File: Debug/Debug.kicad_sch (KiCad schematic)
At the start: 54 parts

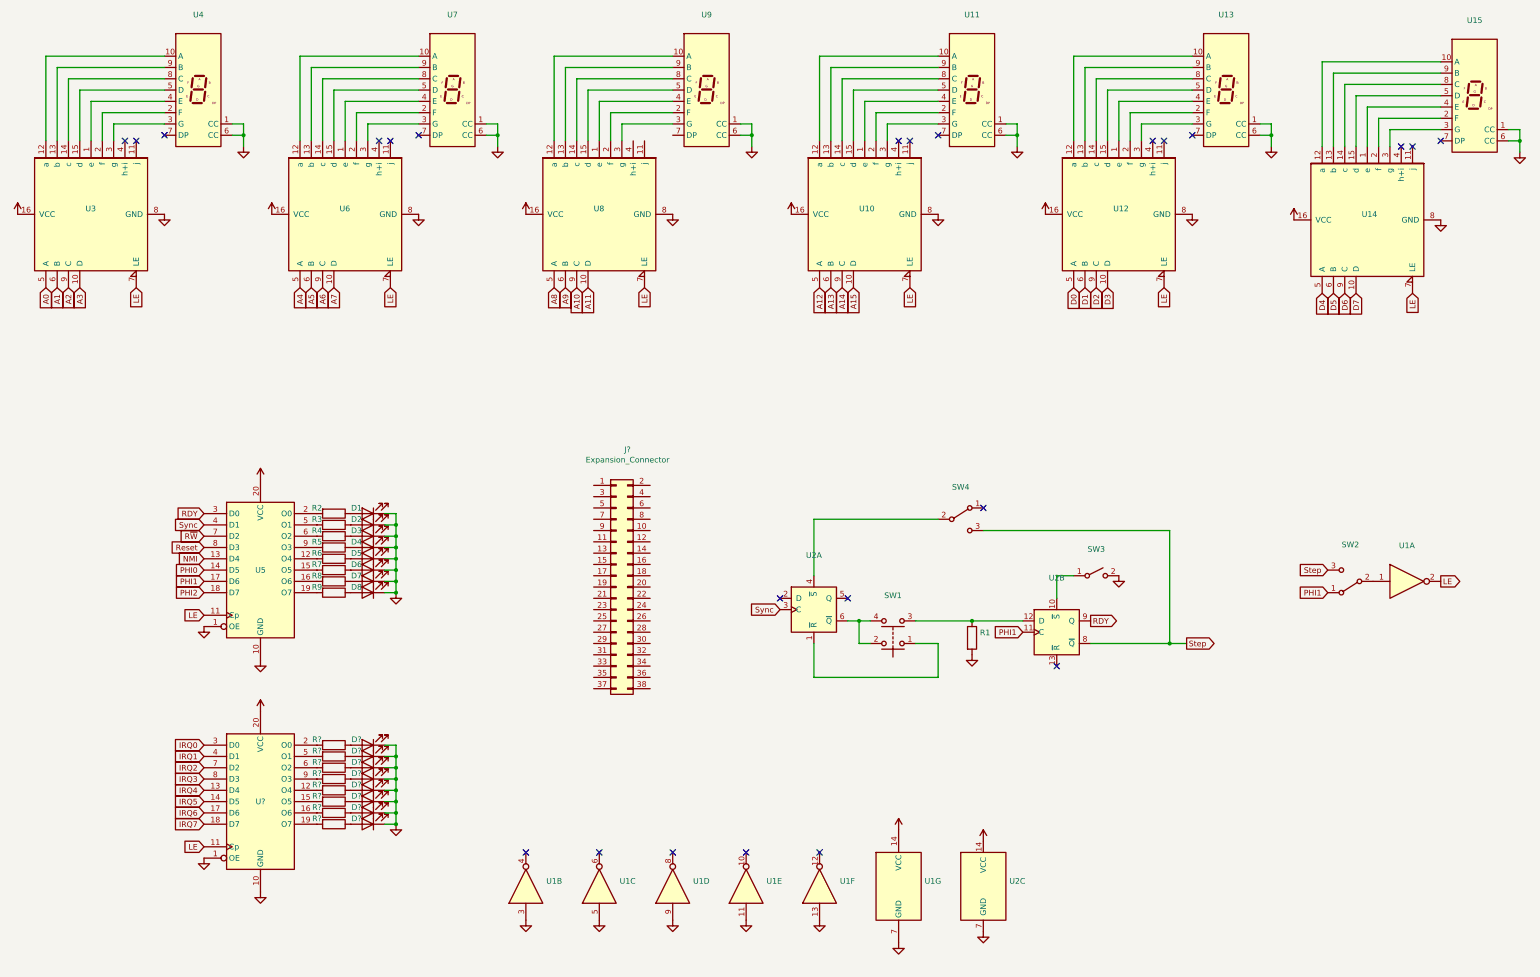
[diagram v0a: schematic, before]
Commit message: Updated debug card...
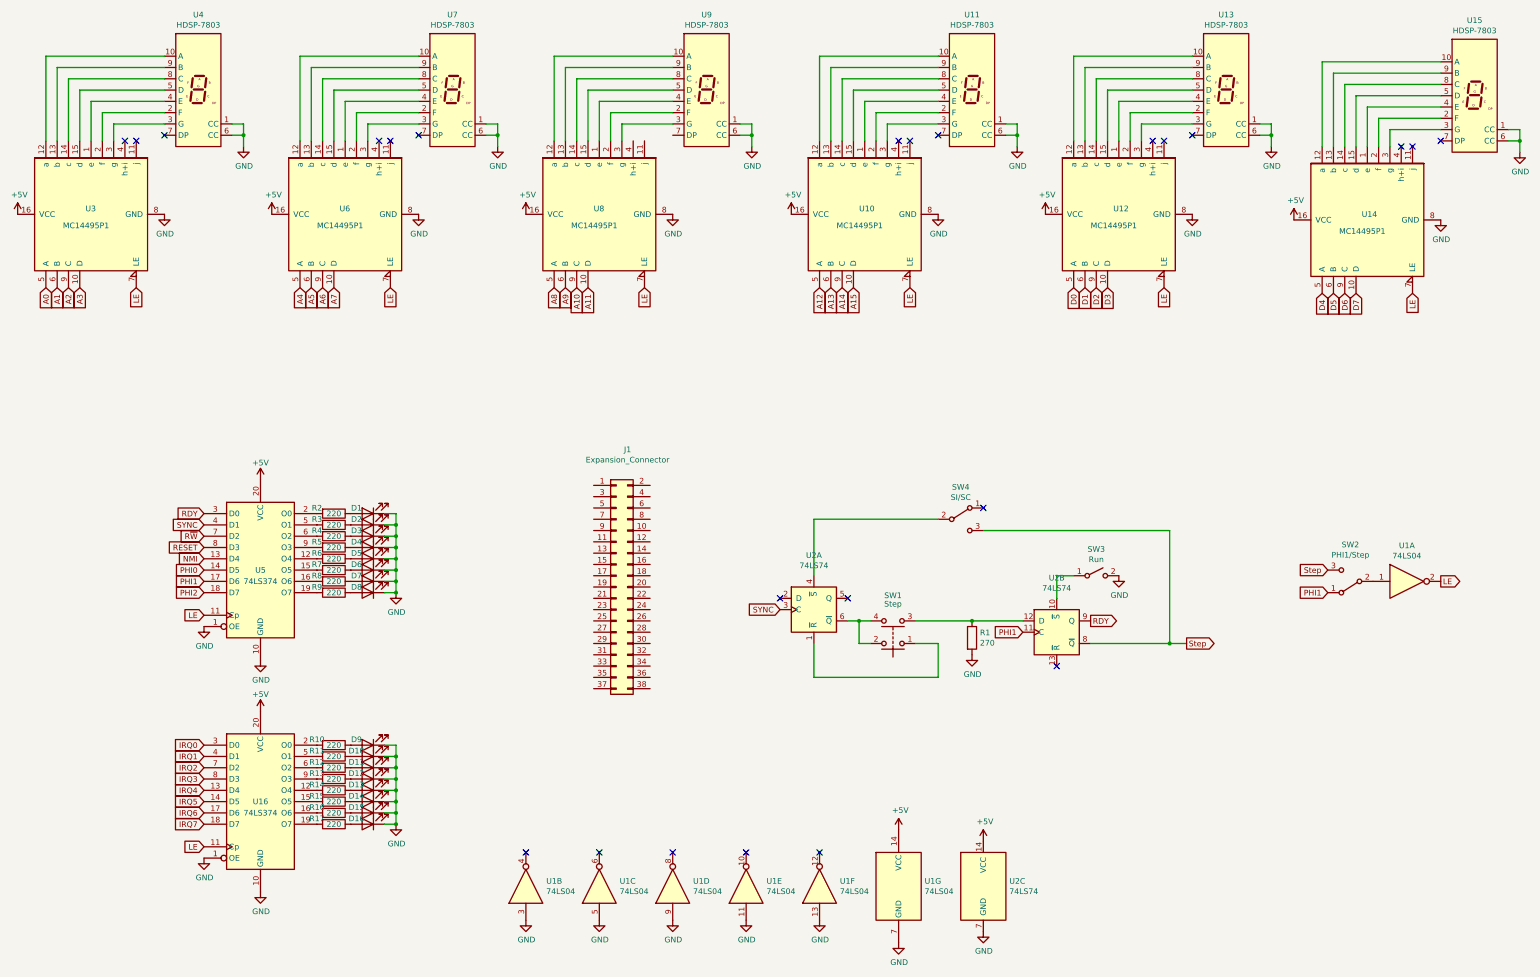
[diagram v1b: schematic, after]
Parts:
- D1: value (none) -> RDY; footprint (none) -> LED_THT:LED_D5.0mm
- D10: renamed from D?; value (none) -> Sync; footprint (none) -> LED_THT:LED_D5.0mm
- D11: renamed from D?; value (none) -> RW; footprint (none) -> LED_THT:LED_D5.0mm
- D12: renamed from D?; value (none) -> Reset; footprint (none) -> LED_THT:LED_D5.0mm
- D13: renamed from D?; value (none) -> IRQ; footprint (none) -> LED_THT:LED_D5.0mm
- D14: renamed from D?; value (none) -> NMI; footprint (none) -> LED_THT:LED_D5.0mm
- D15: renamed from D?; value (none) -> PHI1; footprint (none) -> LED_THT:LED_D5.0mm
- D16: renamed from D?; value (none) -> PHI2; footprint (none) -> LED_THT:LED_D5.0mm
- D2: value (none) -> Sync; footprint (none) -> LED_THT:LED_D5.0mm
- D3: value (none) -> RW; footprint (none) -> LED_THT:LED_D5.0mm
- D4: value (none) -> Reset; footprint (none) -> LED_THT:LED_D5.0mm
- D5: value (none) -> IRQ; footprint (none) -> LED_THT:LED_D5.0mm
- D6: value (none) -> NMI; footprint (none) -> LED_THT:LED_D5.0mm
- D7: value (none) -> PHI1; footprint (none) -> LED_THT:LED_D5.0mm
- D8: value (none) -> PHI2; footprint (none) -> LED_THT:LED_D5.0mm
- D9: renamed from D?; value (none) -> RDY; footprint (none) -> LED_THT:LED_D5.0mm
- R1: value (none) -> 270; footprint (none) -> Resistor_THT:R_Axial_DIN0207_L6.3mm_D2.5mm_P7.62mm_Horizontal
- R10, R11, R12, R13, R14, R15, R16, R17: renamed from R?; value (none) -> 220; footprint (none) -> Resistor_THT:R_Axial_DIN0207_L6.3mm_D2.5mm_P7.62mm_Horizontal
- R2, R3, R4, R5, R6, R7, R8, R9: value (none) -> 220; footprint (none) -> Resistor_THT:R_Axial_DIN0207_L6.3mm_D2.5mm_P7.62mm_Horizontal
- SW1: value (none) -> Step; footprint (none) -> Button_Switch_THT:SW_Push_2P1T_Toggle_CK_PVA1xxH1xxxxxxV2
- SW2: value (none) -> PHI1/Step; footprint (none) -> Button_Switch_THT:SW_Slide_1P2T_CK_OS102011MS2Q
- SW3: value (none) -> Run; footprint (none) -> Button_Switch_THT:SW_DIP_SPSTx01_Slide_9.78x4.72mm_W7.62mm_P2.54mm
- SW4: value (none) -> SI/SC; footprint (none) -> Button_Switch_THT:SW_Slide_1P2T_CK_OS102011MS2Q
- U1: value (none) -> 74LS04; footprint (none) -> Package_DIP:DIP-14_W7.62mm_Socket_LongPads
- U10, U12, U14, U3, U6, U8: value (none) -> MC14495P1; footprint (none) -> Package_DIP:DIP-16_W7.62mm_Socket_LongPads
- U11, U13, U15, U4, U7, U9: value (none) -> HDSP-7803; footprint (none) -> Display_7Segment:HDSP-7801
- U16: renamed from U?; value (none) -> 74LS374; footprint (none) -> Package_DIP:DIP-20_W7.62mm_Socket_LongPads
- U2: value (none) -> 74LS74; footprint (none) -> Package_DIP:DIP-14_W7.62mm_Socket_LongPads
- U5: value (none) -> 74LS374; footprint (none) -> Package_DIP:DIP-20_W7.62mm_Socket_LongPads
- gave numbers to parts that had none: 1
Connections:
- net Reset renamed RESET
- net Sync renamed SYNC
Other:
- company: WolfNet -> WolfNet Computing

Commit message: Debug card layout completed...
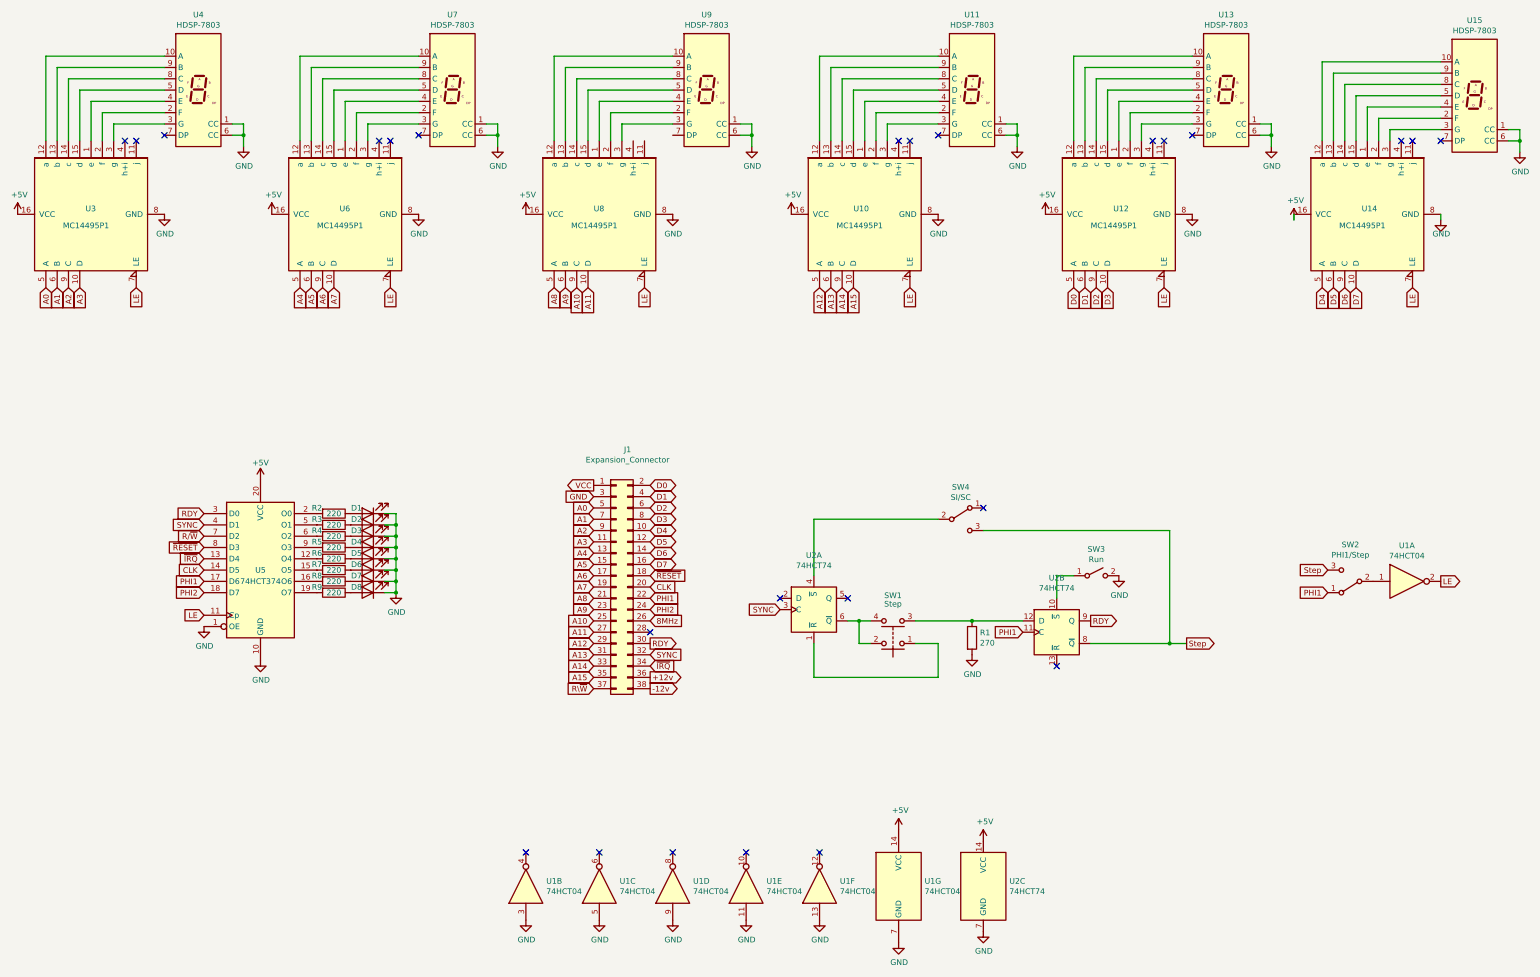
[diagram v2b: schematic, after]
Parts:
- removed D10: Sync, LED_THT:LED_D5.0mm, symbol Debug-rescue:LED-Generic_Device
- removed D11: RW, LED_THT:LED_D5.0mm, symbol Debug-rescue:LED-Generic_Device
- removed D12: Reset, LED_THT:LED_D5.0mm, symbol Debug-rescue:LED-Generic_Device
- removed D13: IRQ, LED_THT:LED_D5.0mm, symbol Debug-rescue:LED-Generic_Device
- removed D14: NMI, LED_THT:LED_D5.0mm, symbol Debug-rescue:LED-Generic_Device
- removed D15: PHI1, LED_THT:LED_D5.0mm, symbol Debug-rescue:LED-Generic_Device
- removed D16: PHI2, LED_THT:LED_D5.0mm, symbol Debug-rescue:LED-Generic_Device
- removed D9: RDY, LED_THT:LED_D5.0mm, symbol Debug-rescue:LED-Generic_Device
- removed R10, R11, R12, R13, R14, R15, R16, R17: 220, Resistor_THT:R_Axial_DIN0207_L6.3mm_D2.5mm_P7.62mm_Horizontal, symbol Debug-rescue:R-Generic_Device
- removed U16: 74LS374, Package_DIP:DIP-20_W7.62mm_Socket_LongPads, symbol 74xx:74LS374
- J1: footprint (none) -> Connector_PinHeader_2.54mm:PinHeader_2x19_P2.54mm_Horizontal
- U1: value 74LS04 -> 74HCT04
- U2: value 74LS74 -> 74HCT74
- U5: value 74LS374 -> 74HCT374
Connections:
- net NMI is gone; now on net ~{IRQ}: U5.13 (D4)
- net PHI0 is gone; now on net CLK: U5.14 (D5)
- net RESET is gone; now on net ~{RESET}: U5.8 (D3)
- net A0: now also J1.5 (Pin_5)
- net A1: now also J1.7 (Pin_7)
- net A10: now also J1.25 (Pin_25)
- net A11: now also J1.27 (Pin_27)
- net A12: now also J1.29 (Pin_29)
- net A13: now also J1.31 (Pin_31)
- net A14: now also J1.33 (Pin_33)
- net A15: now also J1.35 (Pin_35)
- net A2: now also J1.9 (Pin_9)
- net A3: now also J1.11 (Pin_11)
- net A4: now also J1.13 (Pin_13)
- net A5: now also J1.15 (Pin_15)
- net A6: now also J1.17 (Pin_17)
- net A7: now also J1.19 (Pin_19)
- net A8: now also J1.21 (Pin_21)
- net A9: now also J1.23 (Pin_23)
- net D0: now also J1.2 (Pin_2)
- net D1: now also J1.4 (Pin_4)
- net D2: now also J1.6 (Pin_6)
- net D3: now also J1.8 (Pin_8)
- net D4: now also J1.10 (Pin_10)
- net D5: now also J1.12 (Pin_12)
- net D6: now also J1.14 (Pin_14)
- net D7: now also J1.16 (Pin_16)
- net GND: now also J1.3 (Pin_3)
- net PHI1: now also J1.22 (Pin_22)
- net PHI2: now also J1.24 (Pin_24)
- net RDY: now also J1.30 (Pin_30)
- net SYNC: now also J1.32 (Pin_32)
- net VCC: now reaches J1.1
- net ~{RESET}: now reaches J1.18 (Pin_18)
- net CLK: now reaches J1.20 (Pin_20)
- net 8MHz: now reaches J1.26 (Pin_26)
- net ~{IRQ}: now reaches J1.34 (Pin_34)
- net +12v: now reaches J1.36 (Pin_36)
- net R\~{W}: now reaches J1.37 (Pin_37)
- net -12v: now reaches J1.38 (Pin_38)
- net R~{W} renamed R/~{W}
- no-connect marks 24 -> 25
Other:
- moved on the sheet: U14

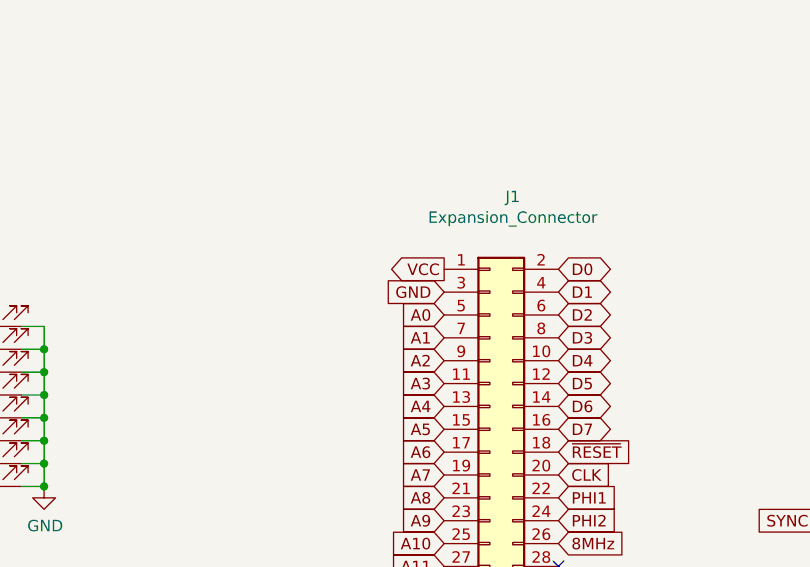
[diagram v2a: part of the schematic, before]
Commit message: 98 unrouted traces...
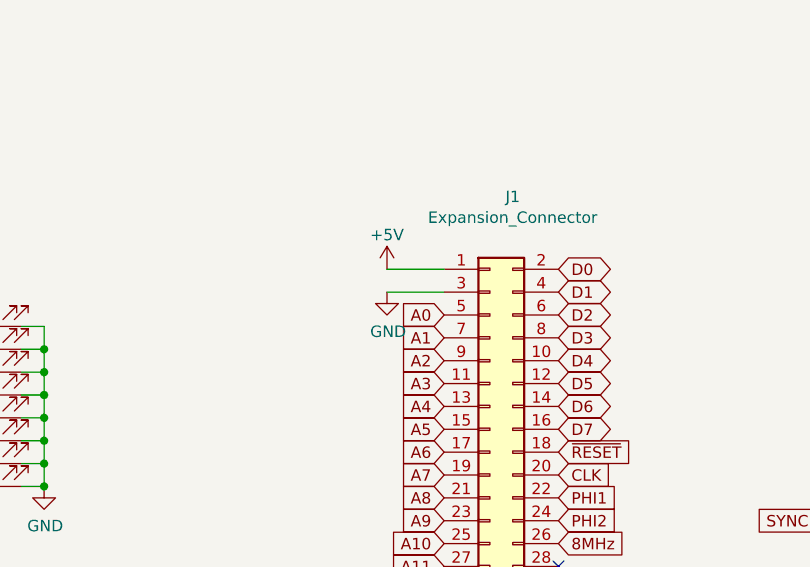
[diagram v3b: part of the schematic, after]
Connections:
- net VCC is gone; now on net +5V: J1.1
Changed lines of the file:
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@@
+    (stroke (width 0) (type default) (color 0 0 0 0))
+  )
+  (wire (pts (xy 149.86 128.27) (xy 156.21 128.27))
     (stroke (width 0) (type default) (color 0 0 0 0))
   )
@@
   )
   (wire (pts (xy 212.09 34.29) (xy 212.09 48.26))
+    (stroke (width 0) (type default) (color 0 0 0 0))
+  )
+  (wire (pts (xy 149.86 125.73) (xy 156.21 125.73))
     (stroke (width 0) (type default) (color 0 0 0 0))
   )
@@
     )
   )
-  (global_label "VCC" (shape output) (at 156.21 125.73 180) (fields_autoplaced)
-    (effects (font (size 1.27 1.27)) (justify right))
-    (property "Intersheet References" "${INTERSHEET_REFS}" (id 0) (at 150.2572 125.6506 0)
-      (effects (font (size 1.27 1.27)) (justify right) hide)
-    )
-  )
   (global_label "A14" (shape input) (at 156.21 166.37 180) (fields_autoplaced)
     (effects (font (size 1.27 1.27)) (justify right))
@@
     (property "Intersheet References" "${INTERSHEET_REFS}" (id 0) (at 0 -1.27 0)
       (effects (font (size 1.27 1.27)) hide)
-    )
-  )
-  (global_label "GND" (shape input) (at 156.21 128.27 180) (fields_autoplaced)
-    (effects (font (size 1.27 1.27)) (justify right))
-    (property "Intersheet References" "${INTERSHEET_REFS}" (id 0) (at 150.0153 128.1906 0)
-      (effects (font (size 1.27 1.27)) (justify right) hide)
     )
   )
@@
     (pin "9")
   )
+  (symbol (lib_id "power:GND") (at 149.86 128.27 0) (unit 1)
+    (in_bom yes) (on_board yes)
+    (property "Reference" "#PWR?" (id 0) (at 149.86 134.62 0)
+      (effects (font (size 1.27 1.27)) hide)
+    )
+    (property "Value" "GND" (id 1) (at 149.987 132.6642 0))
+    (property "Footprint" "" (id 2) (at 149.86 128.27 0)
+      (effects (font (size 1.27 1.27)) hide)
+    )
+    (property "Datasheet" "" (id 3) (at 149.86 128.27 0)
+      (effects (font (size 1.27 1.27)) hide)
+    )
+    (pin "1")
+  )
+  (symbol (lib_id "power:+5V") (at 149.86 125.73 0) (unit 1)
+    (in_bom yes) (on_board yes)
+    (property "Reference" "#PWR?" (id 0) (at 149.86 129.54 0)
+      (effects (font (size 1.27 1.27)) hide)
+    )
+    (property "Value" "+5V" (id 1) (at 149.86 121.92 0))
+    (property "Footprint" "" (id 2) (at 149.86 125.73 0)
+      (effects (font (size 1.27 1.27)) hide)
+    )
+    (property "Datasheet" "" (id 3) (at 149.86 125.73 0)
+      (effects (font (size 1.27 1.27)) hide)
+    )
+    (pin "1")
+  )
   (sheet_instances
     (path "/" (page "1"))
@@
       (reference "#PWR0135") (unit 1) (value "+5V") (footprint "")
     )
+    (path "/1dc9ba2a-69c0-42e3-a4c2-6901de1d5d49"
+      (reference "#PWR?") (unit 1) (value "GND") (footprint "")
+    )
+    (path "/b118dd9e-05e2-402c-8b56-7c9265857475"
+      (reference "#PWR?") (unit 1) (value "+5V") (footprint "")
+    )
     (path "/00000000-0000-0000-0000-00006102ae1c"
